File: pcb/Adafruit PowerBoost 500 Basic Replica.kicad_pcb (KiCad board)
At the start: 2 copper layers, 44 x 32 mm, 31 parts, among them CN1 USBA, J1 HEADER, J2 PWR OUT, J3 Batería, Q1 MMUN2133LT1G, U1 TPS61090RSAR

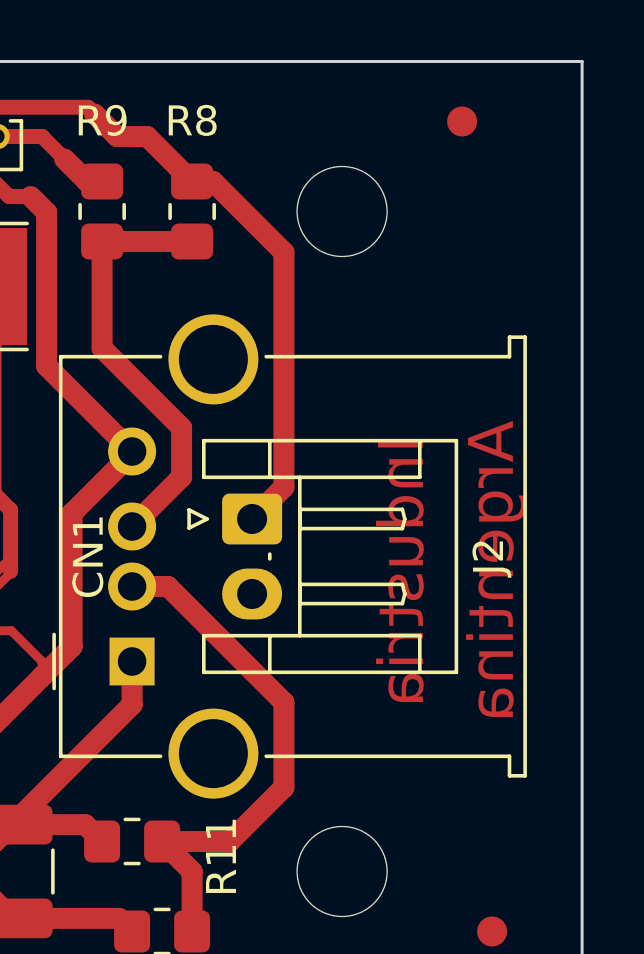
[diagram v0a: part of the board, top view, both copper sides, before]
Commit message: Terminado
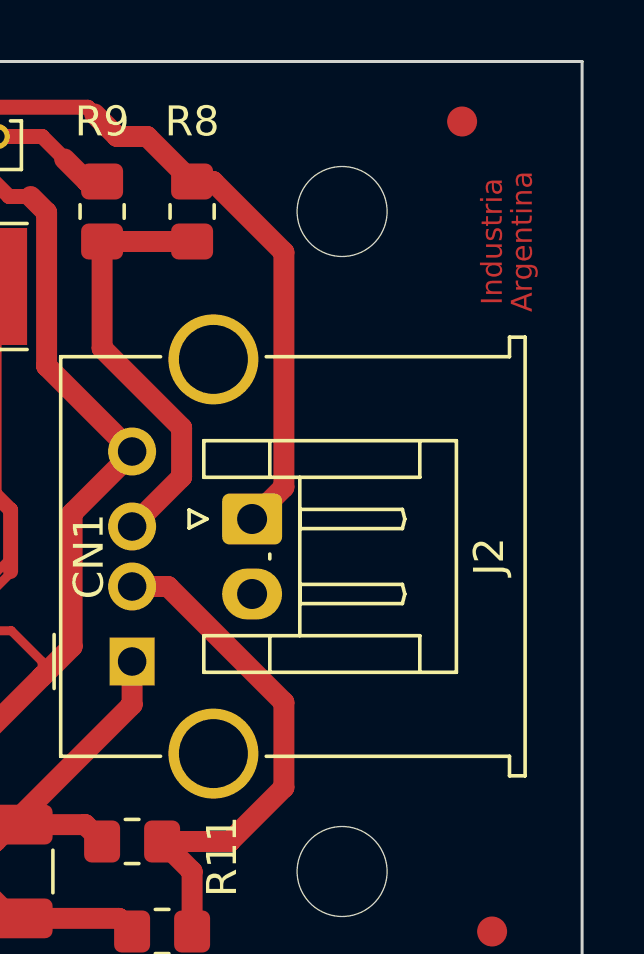
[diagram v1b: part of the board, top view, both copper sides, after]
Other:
- board text added: "Ancho de Pistas: 0.7mm, 0.5mm, 0.3mm"
- board text added: "Clearance 0,3mm"
- board text added: "Espesor 1.6mm"
- board text added: "Espesor de Cobre: 1oz"
- board text added: "Número de Capas: 2"
- board text added: "Terminación superficial: HASL"
- board text added: "Vias 1.6mm/0.8mm"
- board text removed: "Terminación superficial: HASL plomo-estaño"
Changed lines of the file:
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@@
   (general
     (thickness 1.6)
-    (drawings 16)
+    (drawings 37)
     (tracks 192)
     (zones 0)
@@
     )
   )
-  (gr_text Argentina (at 162 107 90) (layer F.Cu)
-    (effects (font (size 1.5 1.5) (thickness 0.3)) (justify mirror))
-  )
-  (gr_text "Industria " (at 159 107 90) (layer F.Cu)
-    (effects (font (size 1.5 1.5) (thickness 0.3)) (justify mirror))
+  (gr_line (start 181 91) (end 182 91) (layer F.CrtYd) (width 0.05))
+  (gr_line (start 181 121) (end 181 91) (layer F.CrtYd) (width 0.05))
+  (gr_line (start 222 121) (end 181 121) (layer F.CrtYd) (width 0.05))
+  (gr_line (start 222 91) (end 222 121) (layer F.CrtYd) (width 0.05))
+  (gr_line (start 221 91) (end 222 91) (layer F.CrtYd) (width 0.05))
+  (gr_line (start 182 91) (end 221 91) (layer F.CrtYd) (width 0.05))
+  (gr_line (start 183 119) (end 183 109) (layer F.CrtYd) (width 0.05))
+  (gr_line (start 220 119) (end 183 119) (layer F.CrtYd) (width 0.05))
+  (gr_line (start 220 109) (end 220 119) (layer F.CrtYd) (width 0.05))
+  (gr_line (start 183 109) (end 220 109) (layer F.CrtYd) (width 0.05))
+  (gr_line (start 183 93) (end 184 93) (layer F.CrtYd) (width 0.05))
+  (gr_line (start 183 105) (end 183 93) (layer F.CrtYd) (width 0.05))
+  (gr_line (start 220 105) (end 183 105) (layer F.CrtYd) (width 0.05))
+  (gr_line (start 220 93) (end 220 105) (layer F.CrtYd) (width 0.05))
+  (gr_line (start 184 93) (end 220 93) (layer F.CrtYd) (width 0.05))
+  (gr_text "Espesor 1.6mm" (at 190.166667 101) (layer F.CrtYd)
+    (effects (font (size 1 1) (thickness 0.15)))
+  )
+  (gr_text "Número de Capas: 2" (at 192.190476 103) (layer F.CrtYd)
+    (effects (font (size 1 1) (thickness 0.15)))
+  )
+  (gr_text "Espesor de Cobre: 1oz" (at 193 99) (layer Dwgs.User)
+    (effects (font (size 1 1) (thickness 0.15)))
+  )
+  (gr_text "Ancho de Pistas: 0.7mm, 0.5mm, 0.3mm" (at 200.095238 117) (layer Dwgs.User)
+    (effects (font (size 1 1) (thickness 0.15)))
+  )
+  (gr_text "Vias 1.6mm/0.8mm" (at 192 115) (layer Dwgs.User)
+    (effects (font (size 1 1) (thickness 0.15)))
+  )
+  (gr_text "Clearance 0,3mm" (at 191.142857 113) (layer Dwgs.User)
+    (effects (font (size 1 1) (thickness 0.15)))
+  )
+  (gr_text Argentina (at 163 96 90) (layer F.Cu)
+    (effects (font (size 0.7 0.7) (thickness 0.175)))
+  )
+  (gr_text "Industria " (at 162 96 90) (layer F.Cu)
+    (effects (font (size 0.7 0.7) (thickness 0.175)))
   )
   (gr_text "Autor: Lucas Orsi" (at 129 120) (layer F.SilkS)
@@
     (effects (font (size 0.6 0.6) (thickness 0.15)))
   )
-  (gr_text "Grillas: 1,000 mm & 0.500 mm" (at 184 95) (layer Dwgs.User)
+  (gr_text "Grillas: 1,000 mm & 0.500 mm" (at 196.666667 111) (layer Dwgs.User)
     (effects (font (size 1 1) (thickness 0.15)))
   )
-  (gr_text "Terminación superficial: HASL plomo-estaño" (at 189 93) (layer Dwgs.User)
+  (gr_text "Terminación superficial: HASL" (at 195.642857 97) (layer Dwgs.User)
     (effects (font (size 1 1) (thickness 0.15)))
   )
-  (gr_text "Fabricante de Referencia: Ernesto Mayer S.A." (at 189 91) (layer Dwgs.User)
+  (gr_text "Fabricante de Referencia: Ernesto Mayer S.A." (at 201.571428 95) (layer Dwgs.User)
     (effects (font (size 1 1) (thickness 0.15)))
   )

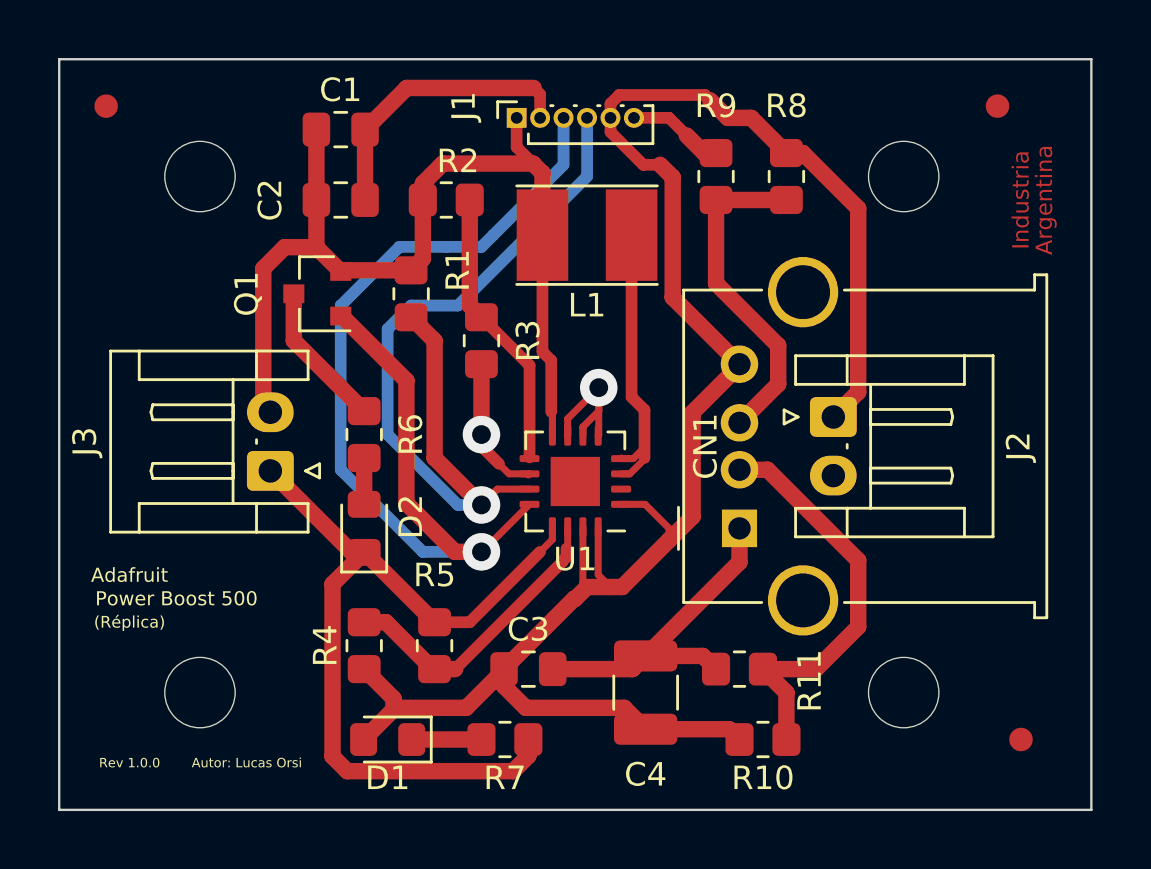
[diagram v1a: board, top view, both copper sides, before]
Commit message: Ultimo commit post presentación
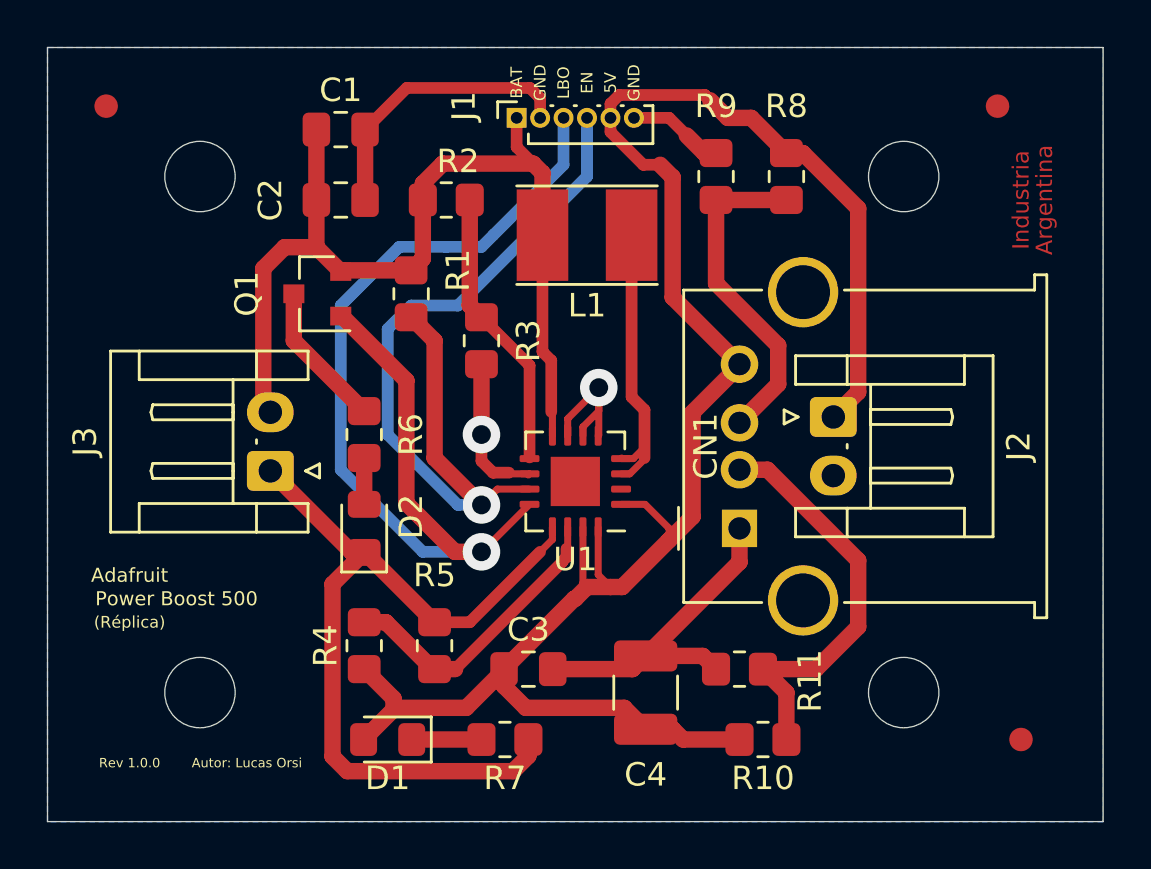
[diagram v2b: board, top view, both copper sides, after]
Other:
- board size 44 x 32 mm -> 45 x 33 mm
- board text added: "5V"
- board text added: "BAT"
- board text added: "EN"
- board text added: "GND"
- board text added: "LBO"
- board text removed: "Espesor de Cobre: 1oz"
- board text removed: "Número de Capas: 2"
